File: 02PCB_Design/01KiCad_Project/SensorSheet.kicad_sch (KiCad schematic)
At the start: 14 parts, among them J1 MTSW-104-22-L-D-265-RA, U1 AS5047P-ATSM, U2 ISM330BXTR

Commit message: Layout progress
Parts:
- C1: footprint Capacitor_SMD:C_0603_1608Metric_Pad1.08x0.95mm_HandSolder -> Package_SO:SOIC-8_3.9x4.9mm_P1.27mm
- J1: footprint (none) -> Connector_PinHeader_2.54mm:PinHeader_2x04_P2.54mm_Horizontal
- U1: footprint (none) -> Package_SO:TSSOP-14_4.4x5mm_P0.65mm
- U2: footprint (none) -> Package_LGA:LGA-14_3x2.5mm_P0.5mm_LayoutBorder3x4y
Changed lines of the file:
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@@
       (effects (font (size 1.27 1.27)))
     )
-    (property "Footprint" "" (at 213.36 74.93 0)
+    (property "Footprint" "Package_SO:TSSOP-14_4.4x5mm_P0.65mm" (at 213.36 74.93 0)
       (effects (font (size 1.27 1.27)) (justify bottom) hide)
     )
@@
       (effects (font (size 1.27 1.27)))
     )
-    (property "Footprint" "" (at 85.09 129.54 0)
+    (property "Footprint" "Connector_PinHeader_2.54mm:PinHeader_2x04_P2.54mm_Horizontal" (at 85.09 129.54 0)
       (effects (font (size 1.27 1.27)) (justify bottom) hide)
     )
@@
       (effects (font (size 1.27 1.27)))
     )
-    (property "Footprint" "" (at 101.6 76.2 0)
+    (property "Footprint" "Package_LGA:LGA-14_3x2.5mm_P0.5mm_LayoutBorder3x4y" (at 101.6 76.2 0)
       (effects (font (size 1.27 1.27)) (justify bottom) hide)
     )
@@
       (effects (font (size 1.27 1.27)) (justify left))
     )
-    (property "Footprint" "Capacitor_SMD:C_0603_1608Metric_Pad1.08x0.95mm_HandSolder" (at 240.9952 68.58 0)
-      (effects (font (size 1.27 1.27)) hide)
-    )
+    (property "Footprint" "Package_SO:SOIC-8_3.9x4.9mm_P1.27mm" (at 240.9952 68.58 0)
+      (effects (font (size 1.27 1.27)) hide)
+    )

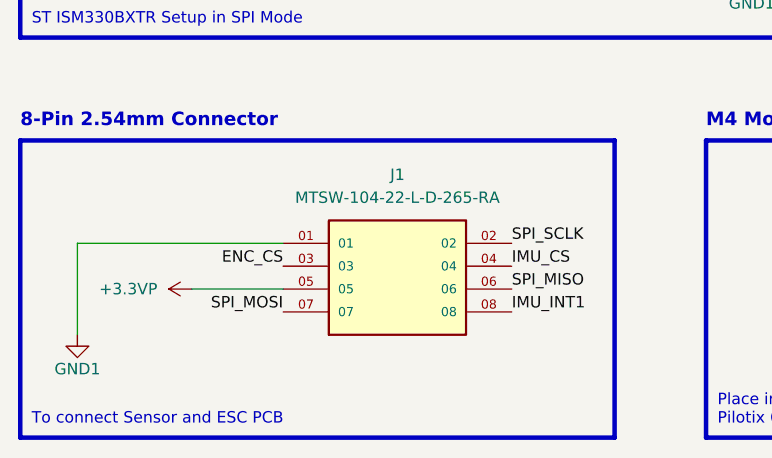
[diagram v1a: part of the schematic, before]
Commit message: Design 1.0 Finished
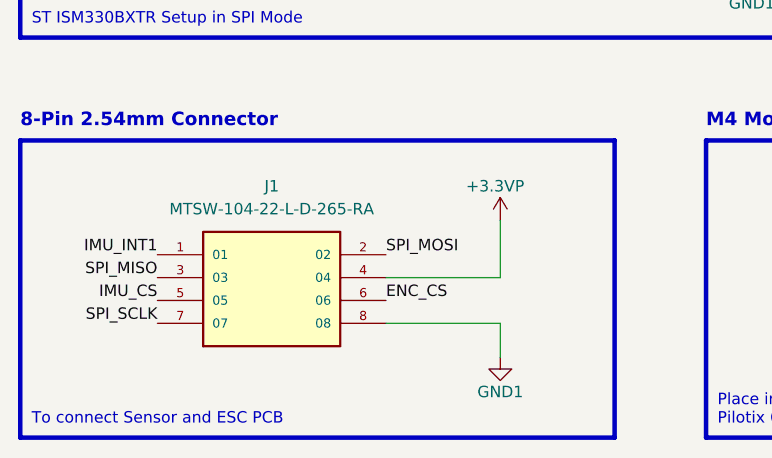
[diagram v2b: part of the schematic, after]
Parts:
- C1: footprint Package_SO:SOIC-8_3.9x4.9mm_P1.27mm -> Capacitor_SMD:C_0603_1608Metric_Pad1.08x0.95mm_HandSolder
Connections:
- net +3.3VP: now also J1.4 (04); no longer J1.05
- net ENC_CS: now also J1.6 (06); no longer J1.03
- net GND1: now also J1.8 (08); no longer J1.01
- net IMU_CS: now also J1.5 (05); no longer J1.04
- net IMU_INT1: now also J1.1 (01); no longer J1.08
- net SPI_MISO: now also J1.3 (03); no longer J1.06
- net SPI_MOSI: now also J1.2 (02); no longer J1.07
- net SPI_SCLK: now also J1.7 (07); no longer J1.02
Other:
- moved on the sheet: J1
